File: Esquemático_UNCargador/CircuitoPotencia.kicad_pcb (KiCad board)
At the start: 2 copper layers, 143.9 x 141 mm, 63 parts, among them IC1 LF353, J1 Conn_01x04_Pin, J2 Relay1, J3 Conn_02x03_Counter_Clockwise, J4 GFCI, J5 PZEM 004T 100A, J6 NTC 3950, J8 Conn_01x02_Pin, J9 Relay2, Q1 PN2222A, Q2 PN2222A, SW1 SW_Push, SW2 SW_Push, SW3 SW_Push, SW4 SW_Push, SW5 SW_Push, U2 LF356, U3 LM7912(Inversor)

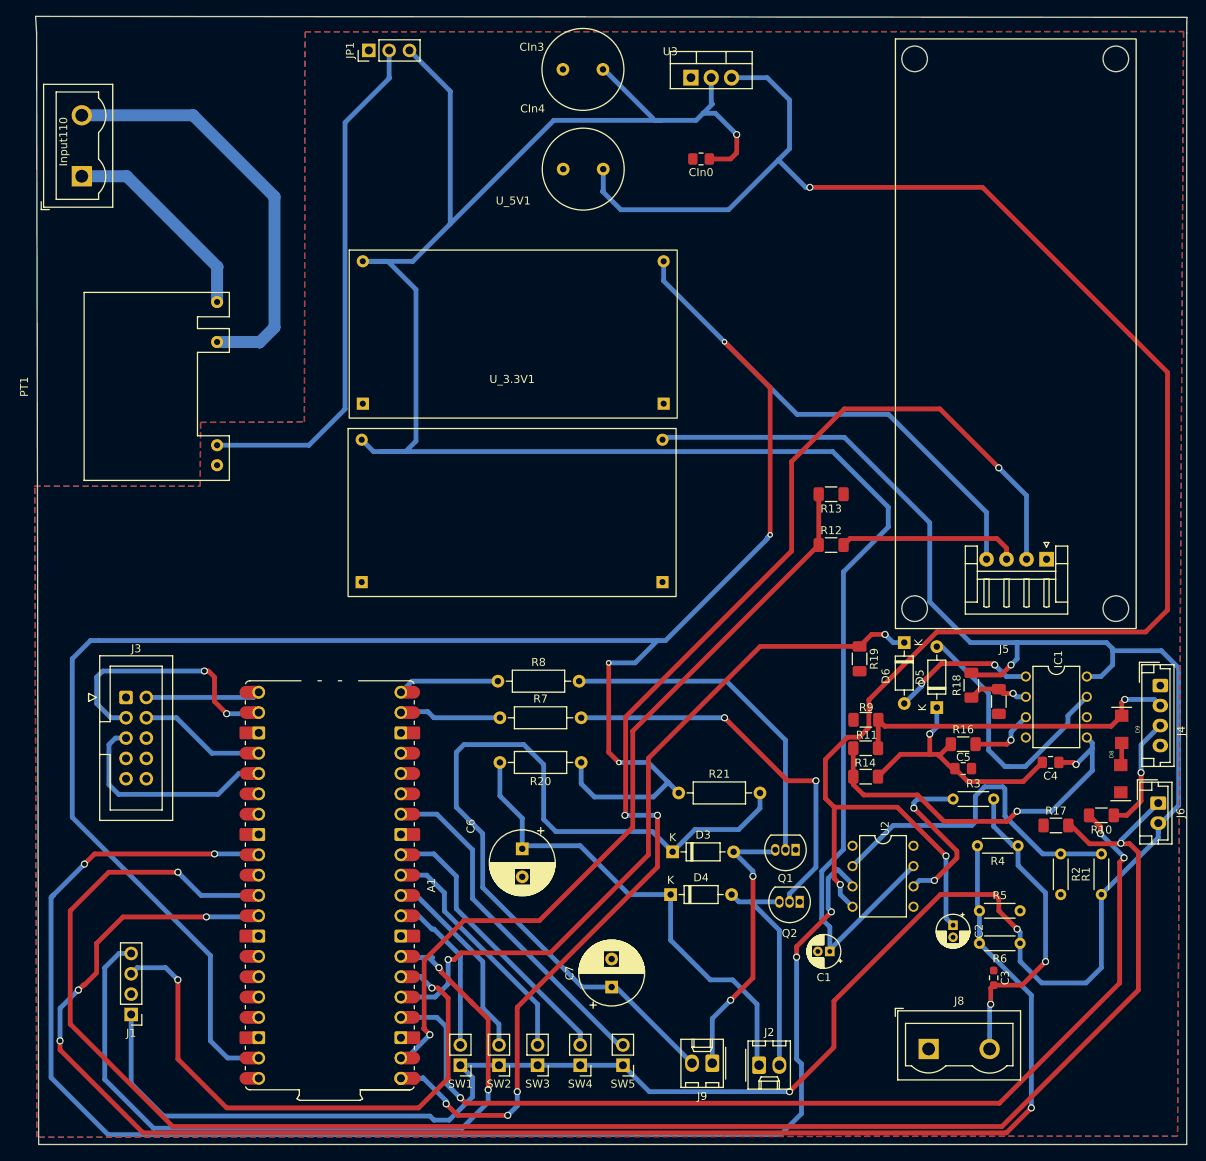
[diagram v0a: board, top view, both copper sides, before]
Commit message: FinalPCB
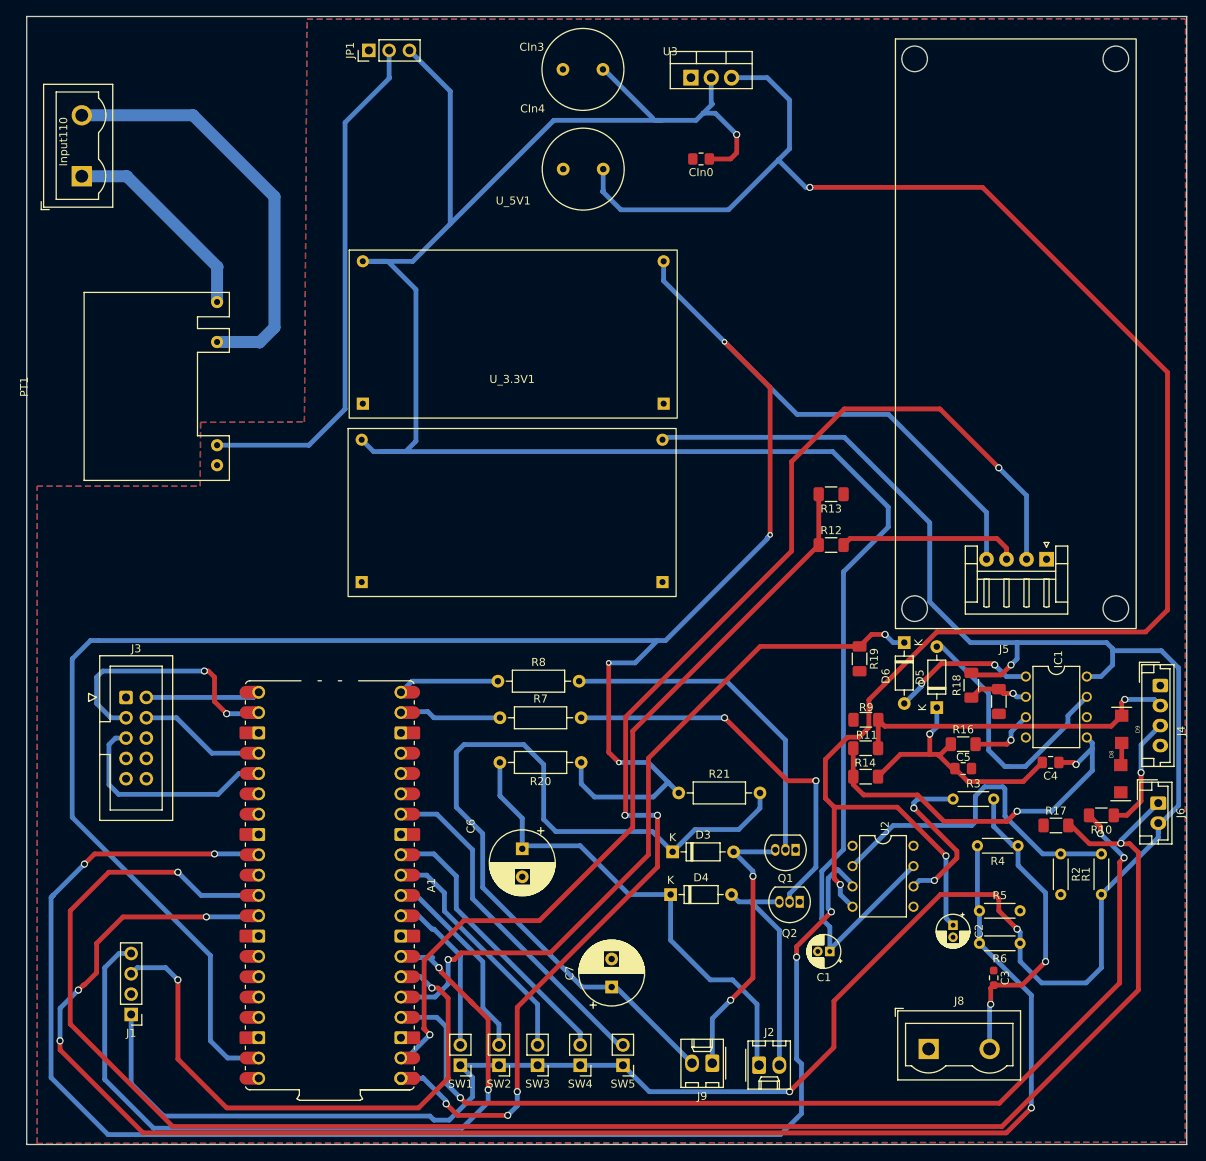
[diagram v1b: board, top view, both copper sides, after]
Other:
- board size 143.9 x 141 mm -> 145 x 141 mm
